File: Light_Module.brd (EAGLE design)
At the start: 63.5 x 88.9 mm, 67 parts, among them IC1 TLC59711, IC2 TLC59711

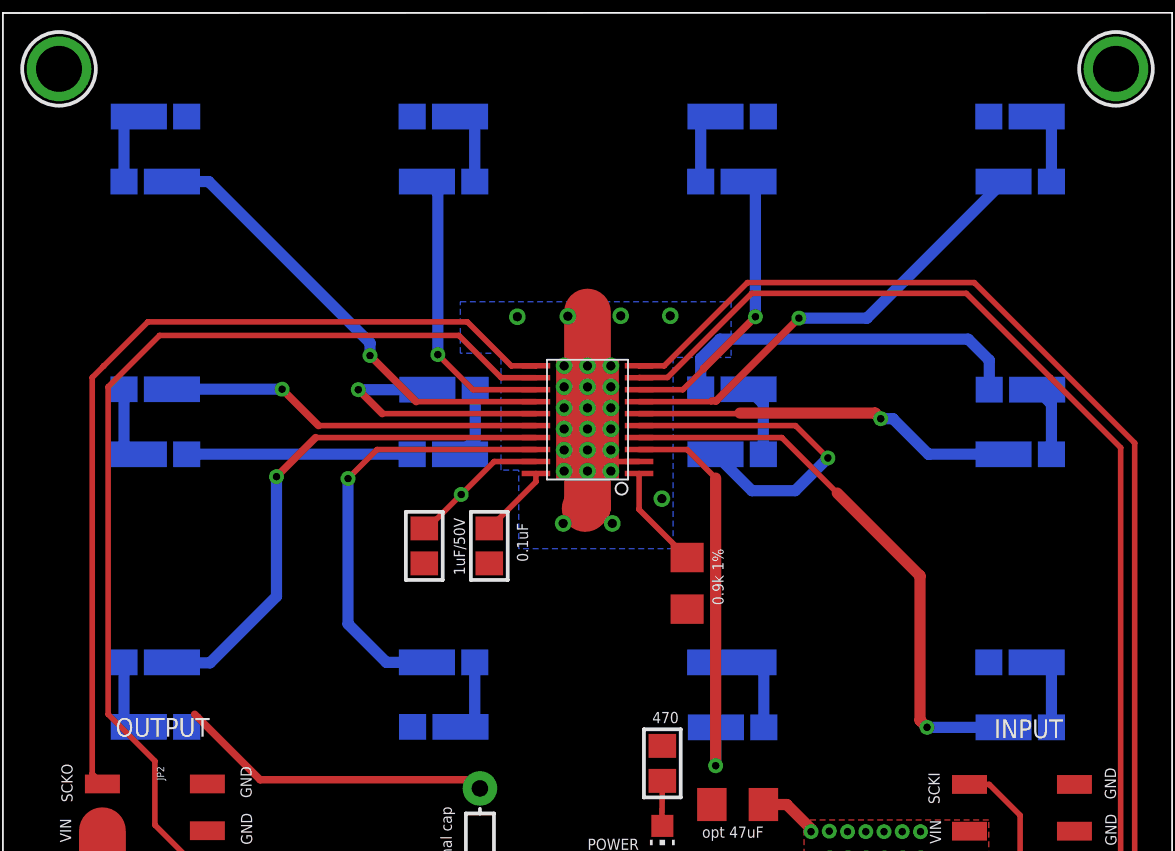
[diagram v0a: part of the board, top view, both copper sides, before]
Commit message: delete some
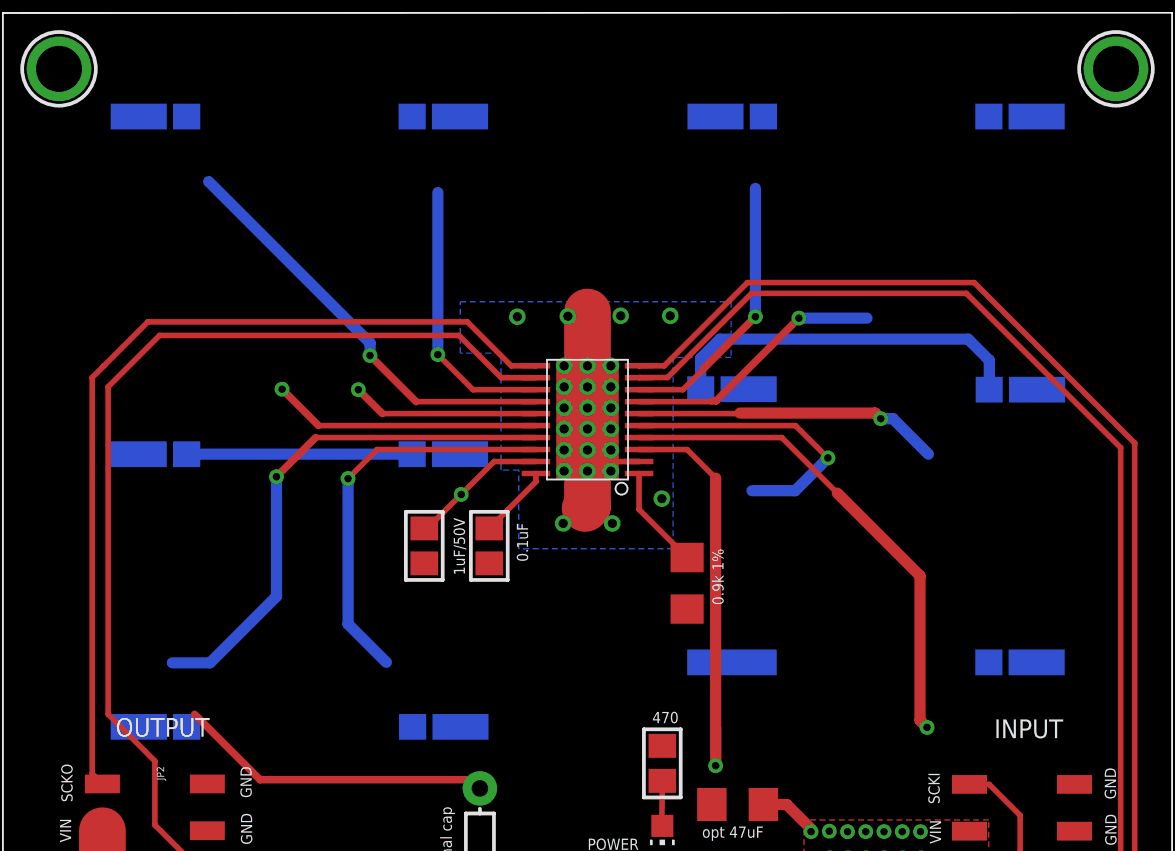
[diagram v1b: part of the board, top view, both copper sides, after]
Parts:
- removed LED27, LED29, LED31, LED33, LED35, LED37, LED39, LED41, LED43, LED45, LED47, LED49: (no value), digikey:DS205
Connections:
- removed net N$20: LED26.P$2, LED27.P$1
- removed net N$21: LED28.P$2, LED29.P$1
- removed net N$22: LED30.P$2, LED31.P$1
- removed net N$23: LED32.P$2, LED33.P$1
- removed net N$24: LED34.P$2, LED35.P$1
- removed net N$25: LED36.P$2, LED37.P$1
- removed net N$26: LED38.P$2, LED39.P$1
- removed net N$27: LED40.P$2, LED41.P$1
- removed net N$28: LED42.P$2, LED43.P$1
- removed net N$29: LED44.P$2, LED45.P$1
- removed net N$30: LED46.P$2, LED47.P$1
- removed net N$31: LED48.P$2, LED49.P$1
- net 2_0: now also LED28.P$2; no longer LED29.P$2
- net 2_1: now also LED26.P$2; no longer LED27.P$2
- net 2_10: now also LED46.P$2; no longer LED47.P$2
- net 2_11: now also LED48.P$2; no longer LED49.P$2
- net 2_2: now also LED32.P$2; no longer LED33.P$2
- net 2_3: now also LED30.P$2; no longer LED31.P$2
- net 2_4: now also LED34.P$2; no longer LED35.P$2
- net 2_5: now also LED36.P$2; no longer LED37.P$2
- net 2_6: now also LED38.P$2; no longer LED39.P$2
- net 2_7: now also LED40.P$2; no longer LED41.P$2
- net 2_8: now also LED42.P$2; no longer LED43.P$2
- net 2_9: now also LED44.P$2; no longer LED45.P$2
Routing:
- net 2_4: track 24.7 -> 14.3 mm
- net 2_9: track 20.6 -> 14.6 mm
- net N$31: track 4.43 -> 0.00 mm
- net N$26: track 4.41 -> 0.00 mm
- net N$24: track 4.39 -> 0.00 mm
- net N$29: track 4.34 -> 0.00 mm
- net N$20: track 4.31 -> 0.00 mm
- net N$27: track 4.30 -> 0.00 mm
- net N$21: track 4.30 -> 0.00 mm
- net N$30: track 4.28 -> 0.00 mm
- net N$25: track 4.24 -> 0.00 mm
- net 2_1: track 30.9 -> 26.8 mm
- net 2_3: track 20.7 -> 16.7 mm
- net N$23: track 3.86 -> 0.00 mm
- net N$28: track 3.85 -> 0.00 mm
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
